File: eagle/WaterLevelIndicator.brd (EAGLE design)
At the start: 62.2 x 78.4 mm, 7 parts, among them IC2 MAX7219CNG

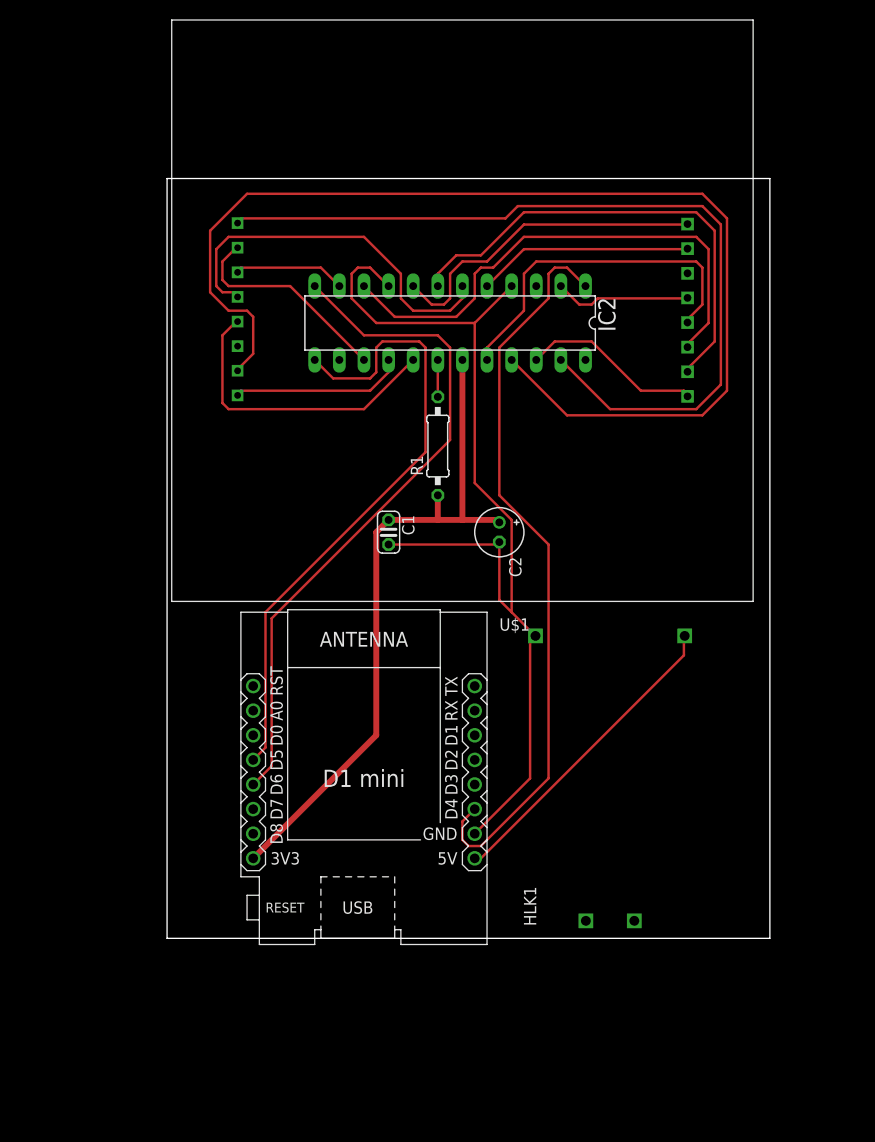
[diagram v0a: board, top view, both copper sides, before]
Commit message: new board
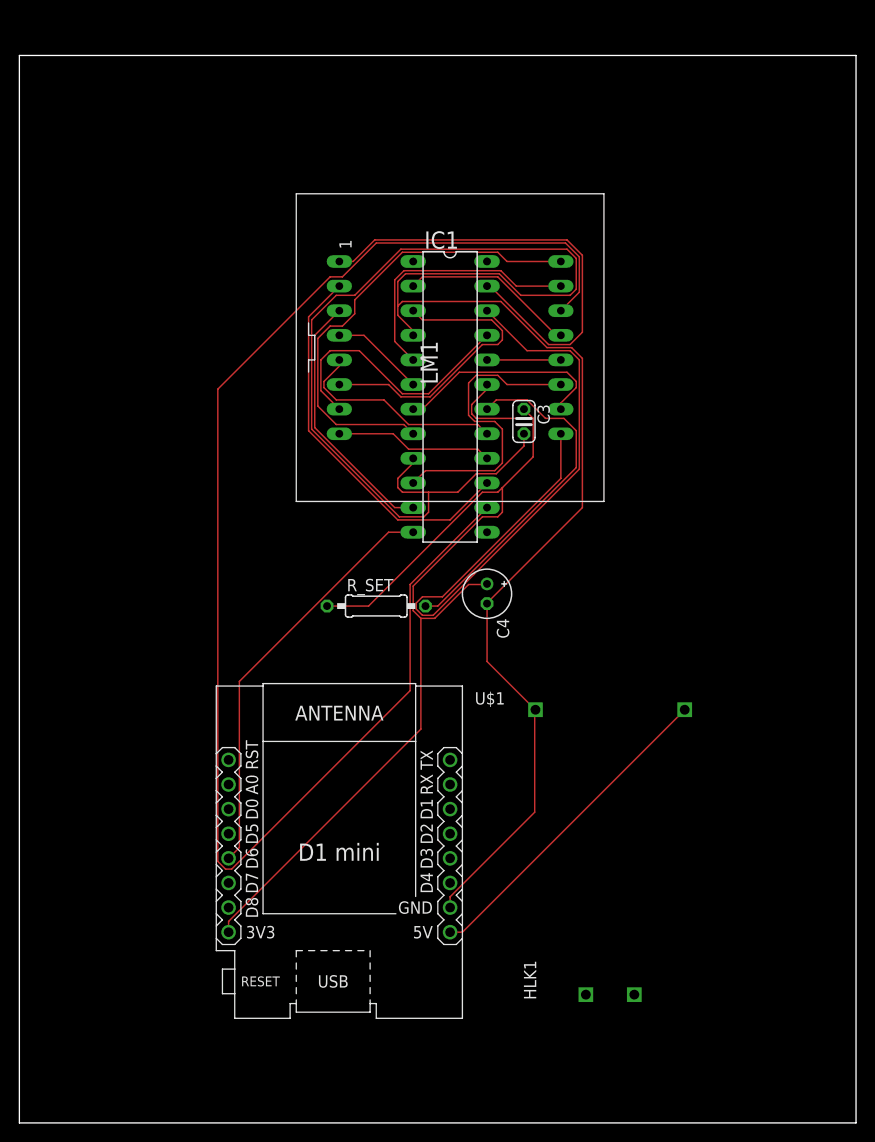
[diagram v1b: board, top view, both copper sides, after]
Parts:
- removed C1: 0.1uF, rcl:C025-024X044
- removed C2: 10uF, rcl:E2-5
- removed IC2: MAX7219CNG, maxim:DIL24-3
- removed R1: 62K, resistor:0207/10
- removed U$3: 8X8-LED-MATRIX, 8 X 8 LED Matrix:8X8-LED-MATRIX
- added C3: 0.1uF, rcl:C025-024X044
- added C4: 10uF, rcl:E2-5
- added IC1: MAX7219CNG, maxim:DIL24-3
- added LM1: LED MATRIX, MajicDesigns:LED_MATRIX
- added R_SET: 62k, rcl:0207/10
- moved U$1 8.03 mm to (12.7, 33.0)
- moved HLK1 7.62 mm to (40.6, 33.0)
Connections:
- removed net N$1: C1.2, C2.-, HLK1.P$3, IC2.4, IC2.9, U$1.JP2.7
- removed net N$12: IC2.2, U$3.P$13
- removed net N$13: IC2.11, U$3.P$3
- removed net N$14: IC2.6, U$3.P$4
- removed net N$15: IC2.7, U$3.P$10
- removed net N$16: IC2.3, U$3.P$6
- removed net N$17: IC2.10, U$3.P$11
- removed net N$18: IC2.5, U$3.P$15
- removed net N$19: IC2.8, U$3.P$16
- removed net N$20: IC2.14, U$3.P$14
- removed net N$21: IC2.16, U$3.P$8
- removed net N$22: IC2.20, U$3.P$12
- removed net N$23: IC2.23, U$3.P$1
- removed net N$24: IC2.21, U$3.P$7
- removed net N$25: IC2.15, U$3.P$2
- removed net N$26: IC2.17, U$3.P$5
- removed net N$27: IC2.22, U$3.P$9
- removed net N$28: C1.1, C2.+, IC2.19, R1.1, U$1.JP1.8
- removed net N$7: IC2.18, R1.2
- new net GND: C3.2, C4.-, HLK1.P$3, IC1.4, IC1.9, U$1.JP2.7
- new net N$10: IC1.20, LM1.12
- new net N$11: IC1.16, LM1.8
- new net N$29: IC1.14, LM1.14
- new net N$3: IC1.15, LM1.2
- new net N$30: IC1.22, LM1.9
- new net N$31: IC1.8, LM1.16
- new net N$32: IC1.5, LM1.15
- new net N$33: IC1.10, LM1.11
- new net N$34: IC1.3, LM1.6
- new net N$35: IC1.7, LM1.10
- new net N$36: IC1.6, LM1.4
- new net N$37: IC1.11, LM1.3
- new net N$38: IC1.2, LM1.13
- new net N$43: IC1.18, R_SET.2
- new net N$44: IC1.17, LM1.5
- new net N$8: IC1.21, LM1.7
- new net N$9: IC1.23, LM1.1
- new net VCC: C3.1, C4.+, IC1.19, R_SET.1, U$1.JP1.8
- net N$4: now also IC1.1; no longer IC2.1
- net N$5: now also IC1.12; no longer IC2.12
- net N$6: now also IC1.13; no longer IC2.13
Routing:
- net GND: track 0.00 -> 197.7 mm
- net N$29: track 0.00 -> 149.2 mm
- net N$24: track 117.4 -> 0.00 mm
- net VCC: track 0.00 -> 110.7 mm
- net N$1: track 103.9 -> 0.00 mm
- net N$23: track 87.6 -> 0.00 mm
- net N$4: track 76.9 -> 0.00 mm
- net N$30: track 0.00 -> 71.7 mm
- net N$28: track 71.4 -> 0.00 mm
- net N$6: track 65.5 -> 0.00 mm
- net N$17: track 53.3 -> 0.00 mm
- net N$15: track 48.9 -> 0.00 mm
- net N$31: track 0.00 -> 48.0 mm
- net N$9: track 0.00 -> 47.5 mm
- net N$3: track 0.00 -> 40.0 mm
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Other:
- board size 62.2 x 78.4 mm -> 86.3 x 110.2 mm
